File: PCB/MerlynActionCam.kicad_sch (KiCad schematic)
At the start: 65 parts, among them Q1 AO3401A, Q2 AO3401A, Q3 AO3401A, SW1 TS24CA, U1 TPS63802DLAR, U2 BQ25606RGER, U3 RT8097CHGE, U4 RT8097CHGE, U5 CH32V003F4U6

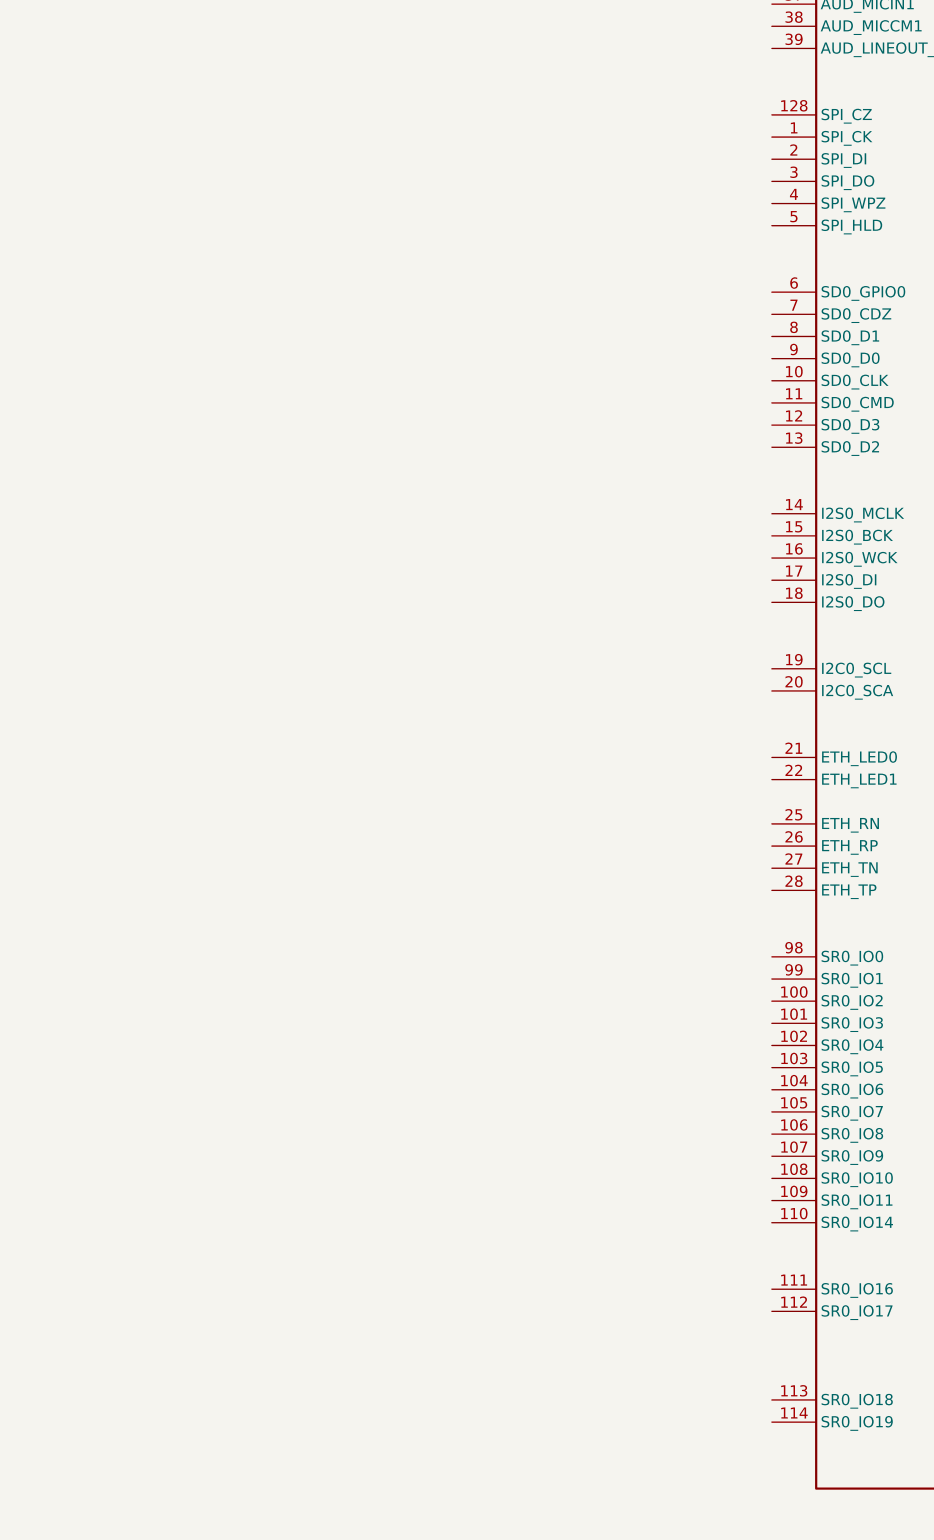
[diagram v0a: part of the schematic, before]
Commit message: checkpoint
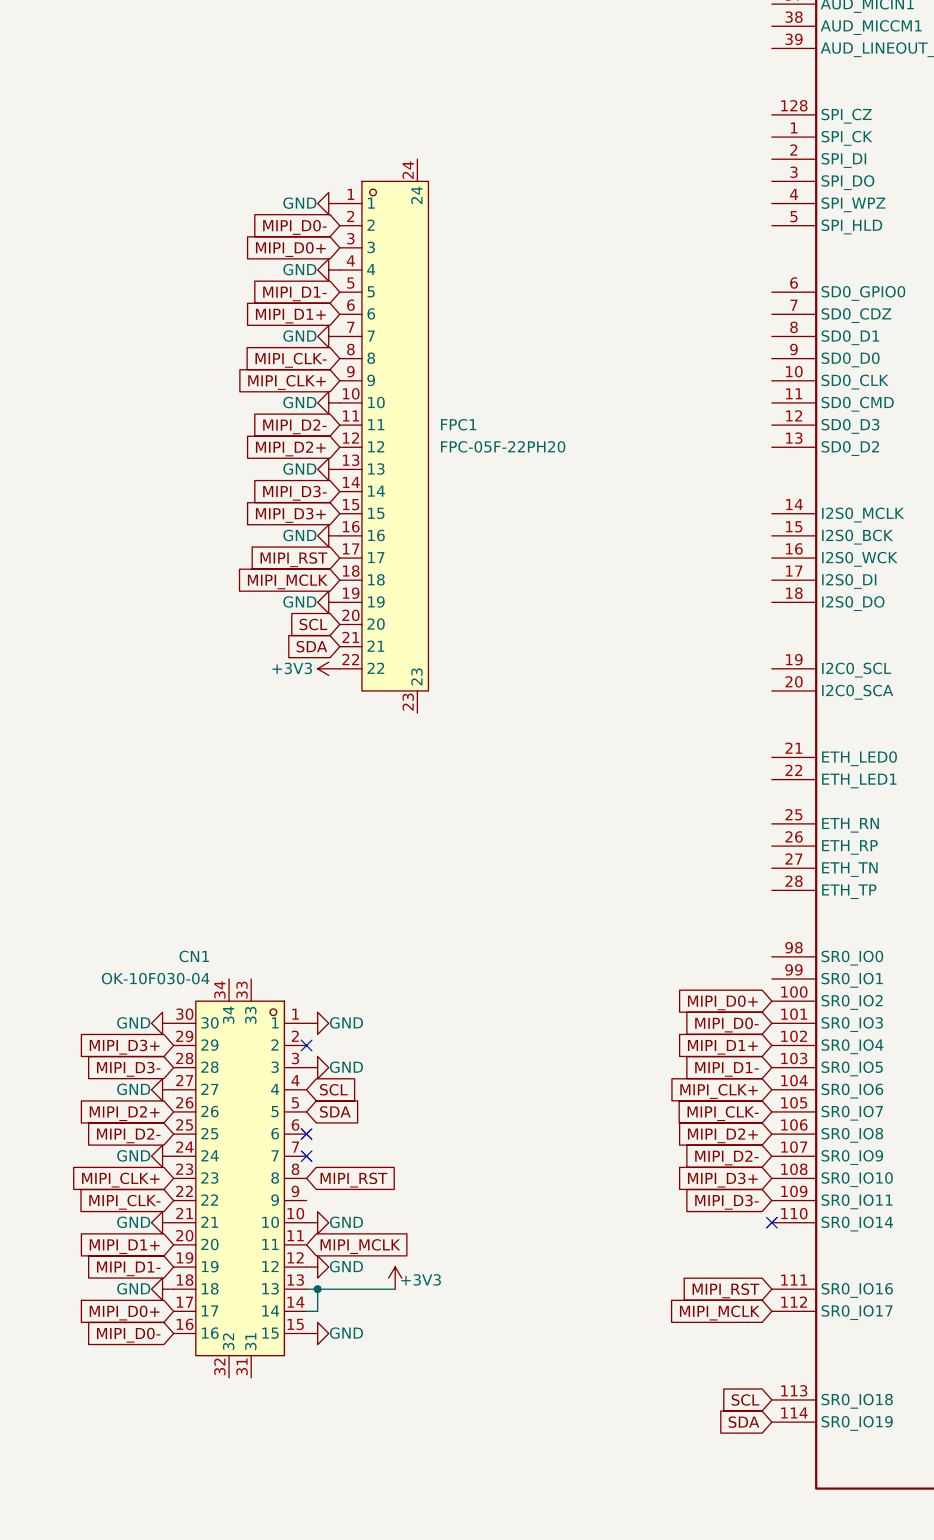
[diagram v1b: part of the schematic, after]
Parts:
- added CN1: OK-10F030-04, easyeda2kicad:CONN-SMD_30P-P0.40_OK-10F030-04-A, symbol MerlynActionCam:OK-10F030-04
- added FPC1: FPC-05F-22PH20, easyeda2kicad:FPC-SMD_22P-P0.50_FPC-05F-22PH20, symbol MerlynActionCam:FPC-05F-22PH20
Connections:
- net +3V3: now also CN1.13, CN1.14, FPC1.22
- net GND: now also CN1.1, CN1.10, CN1.12, CN1.15, CN1.18, CN1.21, CN1.24, CN1.27, CN1.3, CN1.30, FPC1.1, FPC1.10, FPC1.13, FPC1.16, FPC1.19, FPC1.4, FPC1.7
- net MIPI_D0+: now reaches 1.100 (SR0_IO2)
- net MIPI_D0+: now also CN1.17, FPC1.3
- net MIPI_D0-: now reaches 1.101 (SR0_IO3)
- net MIPI_D0-: now also CN1.16, FPC1.2
- net MIPI_D1+: now reaches 1.102 (SR0_IO4)
- net MIPI_D1+: now also CN1.20, FPC1.6
- net MIPI_D1-: now reaches 1.103 (SR0_IO5)
- net MIPI_D1-: now also CN1.19, FPC1.5
- net MIPI_CLK+: now reaches 1.104 (SR0_IO6)
- net MIPI_CLK+: now also CN1.23, FPC1.9
- net MIPI_CLK-: now reaches 1.105 (SR0_IO7)
- net MIPI_CLK-: now also CN1.22, FPC1.8
- net MIPI_D2+: now reaches 1.106 (SR0_IO8)
- net MIPI_D2+: now also CN1.26, FPC1.12
- net MIPI_D2-: now reaches 1.107 (SR0_IO9)
- net MIPI_D2-: now also CN1.25, FPC1.11
- net MIPI_D3+: now reaches 1.108 (SR0_IO10)
- net MIPI_D3+: now also CN1.29, FPC1.15
- net MIPI_D3-: now reaches 1.109 (SR0_IO11)
- net MIPI_D3-: now also CN1.28, FPC1.14
- net MIPI_RST: now reaches 1.111 (SR0_IO16)
- net MIPI_RST: now also CN1.8, FPC1.17
- net MIPI_MCLK: now reaches 1.112 (SR0_IO17)
- net MIPI_MCLK: now also CN1.11, FPC1.18
- net SCL: now reaches 1.113 (SR0_IO18)
- net SCL: now also CN1.4, FPC1.20
- net SDA: now reaches 1.114 (SR0_IO19)
- net SDA: now also CN1.5, FPC1.21
- no-connect marks 17 -> 21
